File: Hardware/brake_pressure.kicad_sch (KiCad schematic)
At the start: 12 parts, among them U11 MCP6002-xSN

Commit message: Changes in CAN section
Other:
- title: (none) -> FrontBox
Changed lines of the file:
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@@
 	(generator_version "9.0")
 	(paper "A4")
+	(title_block
+		(title "FrontBox")
+	)
 	(junction
 		(at 91.44 50.8)

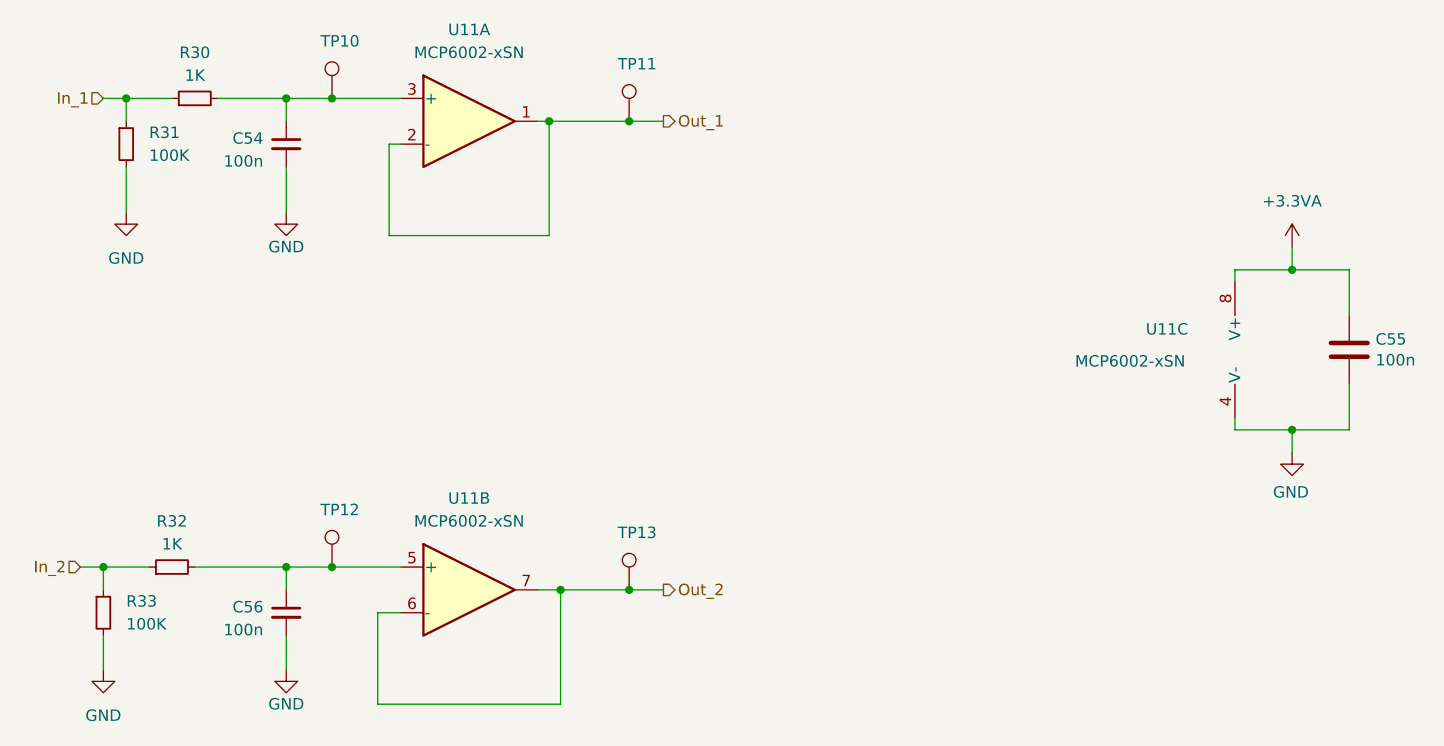
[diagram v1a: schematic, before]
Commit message: BOM update
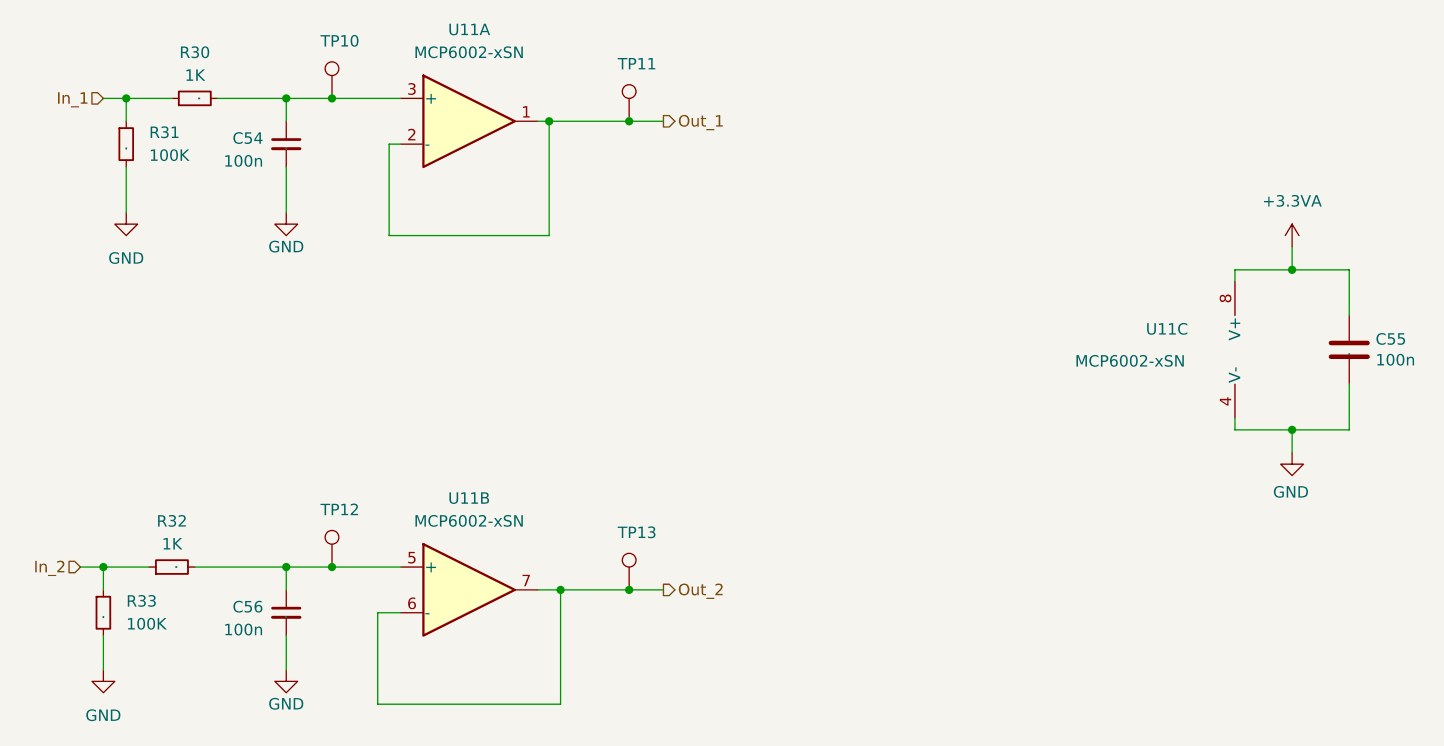
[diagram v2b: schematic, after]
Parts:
- C54, C55, C56, R30, R31, R32, R33: Mouser Part Number (none) -> .
- U11: Mouser Part Number (none) -> 579-MCP6002-E/SN
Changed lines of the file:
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@@
+			)
+		)
+		(property "Mouser Part Number" "."
+			(at 86.36 55.88 0)
+			(effects
+				(font
+					(size 1.27 1.27)
+				)
 			)
 		)
@@
 			)
 		)
+		(property "Mouser Part Number" "."
+			(at 66.04 107.95 0)
+			(effects
+				(font
+					(size 1.27 1.27)
+				)
+			)
+		)
 		(pin "2"
 		)
@@
 			)
 		)
+		(property "Mouser Part Number" "."
+			(at 68.58 55.88 0)
+			(effects
+				(font
+					(size 1.27 1.27)
+				)
+			)
+		)
 		(pin "2"
 		)
@@
 			)
 		)
+		(property "Mouser Part Number" "."
+			(at 86.36 107.95 0)
+			(effects
+				(font
+					(size 1.27 1.27)
+				)
+			)
+		)
 		(pin "1"
 		)
@@
 			)
 		)
+		(property "Mouser Part Number" "579-MCP6002-E/SN"
+			(at 106.68 105.41 0)
+			(effects
+				(font
+					(size 1.27 1.27)
+				)
+				(hide yes)
+			)
+		)
 		(pin "2"
 		)
@@
 			)
 		)
+		(property "Mouser Part Number" "579-MCP6002-E/SN"
+			(at 106.68 53.34 0)
+			(effects
+				(font
+					(size 1.27 1.27)
+				)
+				(hide yes)
+			)
+		)
 		(pin "2"
 		)
@@
 				)
 				(hide yes)
+			)
+		)
+		(property "Mouser Part Number" "."
+			(at 204.47 78.74 0)
+			(effects
+				(font
+					(size 1.27 1.27)
+				)
 			)
 		)
@@
 			)
 		)
+		(property "Mouser Part Number" "579-MCP6002-E/SN"
+			(at 194.31 78.74 0)
+			(effects
+				(font
+					(size 1.27 1.27)
+				)
+				(hide yes)
+			)
+		)
 		(pin "2"
 		)
@@
 			)
 		)
+		(property "Mouser Part Number" "."
+			(at 76.2 50.8 0)
+			(effects
+				(font
+					(size 1.27 1.27)
+				)
+			)
+		)
 		(pin "2"
 		)
@@
 			)
 		)
+		(property "Mouser Part Number" "."
+			(at 73.66 102.87 0)
+			(effects
+				(font
+					(size 1.27 1.27)
+				)
+			)
+		)
